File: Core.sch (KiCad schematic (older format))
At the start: 2 parts

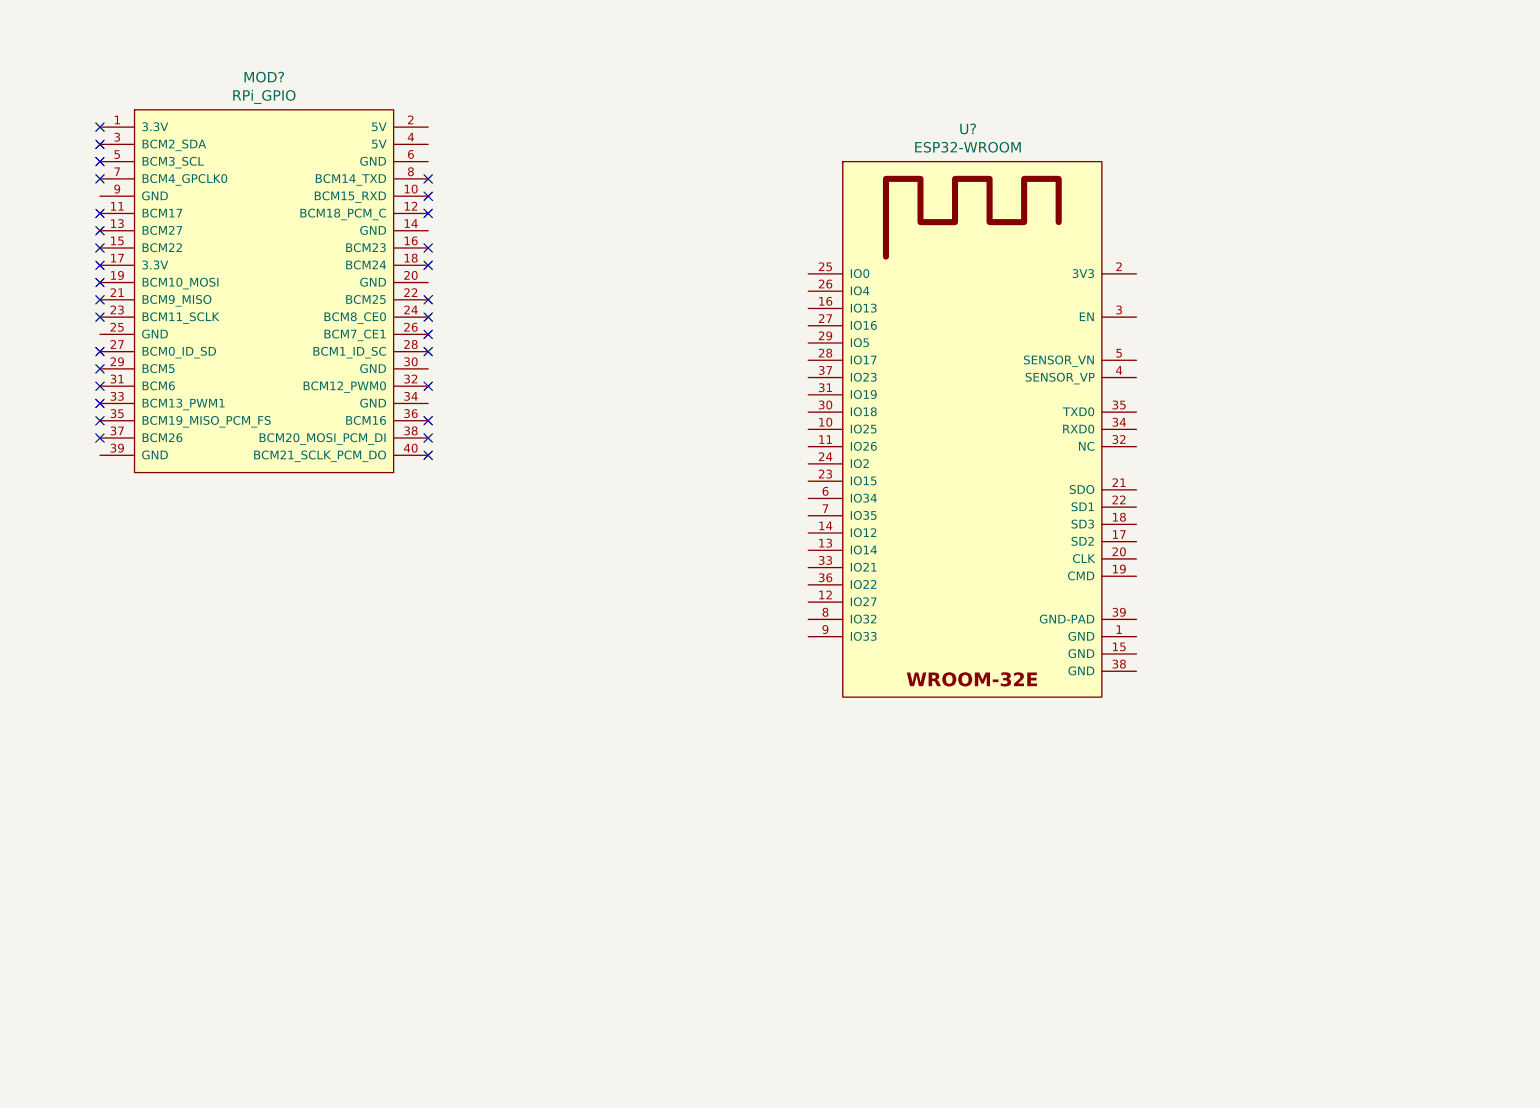
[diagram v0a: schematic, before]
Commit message: Agrego v1.0 de SmartSaffron
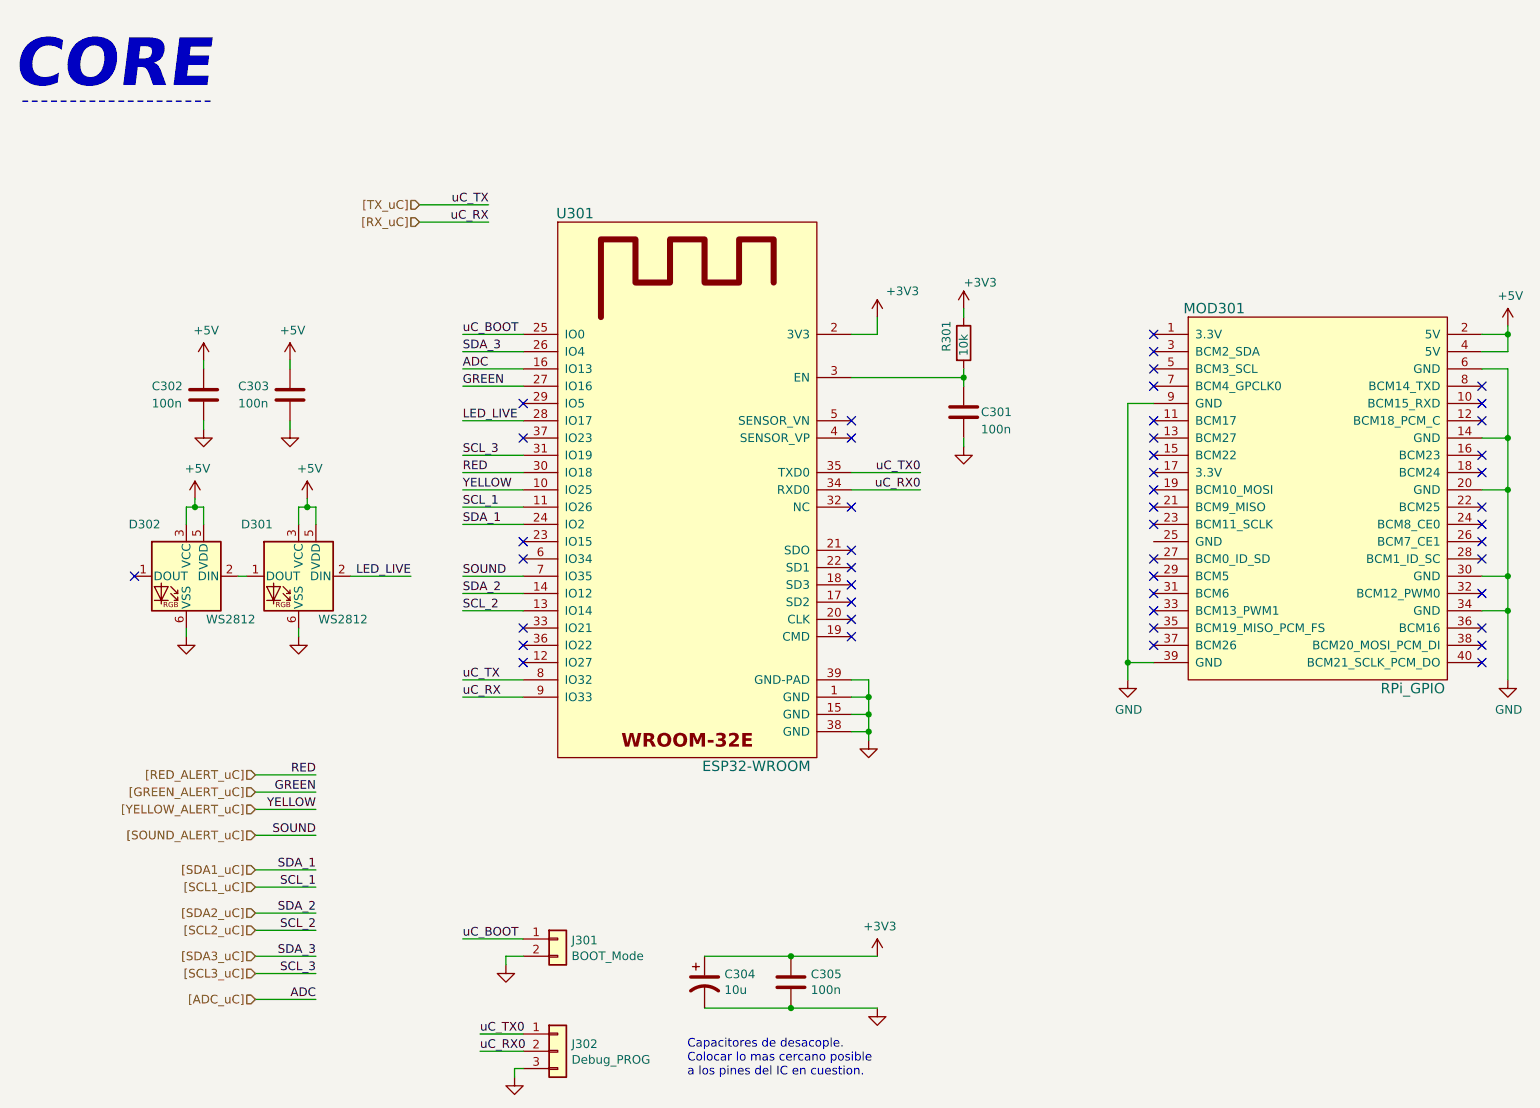
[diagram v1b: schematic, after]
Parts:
- added C301, C302, C303, C305: 100n, 00_lib_fp:C_0805_2012Metric_Pad1.18x1.45mm_HandSolder, symbol 00_lib_sch:C
- added C304: 10u, 00_lib_fp:C_0805_2012Metric_Pad1.18x1.45mm_HandSolder, symbol 00_lib_sch:CP1
- added D301, D302: WS2812, 00_lib_fp:LED_WS2812_PLCC6_5.0x5.0mm_P1.6mm, symbol 00_lib_sch:WS2812
- added J301: BOOT_Mode, 00_lib_fp:PinHeader_1x02_P2.54mm_Vertical, symbol 00_lib_sch:Conn_01x02
- added J302: Debug_PROG, 00_lib_fp:PinHeader_1x03_P2.54mm_Vertical, symbol Connector_Generic:Conn_01x03
- added R301: 10k, 00_lib_fp:R_0805_2012Metric_Pad1.20x1.40mm_HandSolder, symbol 00_lib_sch:R
- MOD301: renamed from MOD?; footprint 00_lib_fp:RPi_fp -> 00_lib_fp:PinSocket_2x20_P2.54mm_Vertical_SMD
- gave numbers to parts that had none: 1
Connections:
- net GND: now reaches MOD301.14 (GND)
- net GND: now also MOD301.20 (GND), MOD301.30 (GND), MOD301.34 (GND), MOD301.39 (GND), MOD301.6 (GND), MOD301.9 (GND), U301.1 (GND), U301.15 (GND), U301.38 (GND), U301.39 (GND-PAD), C301.2, C302.2, C303.2, C304.2, C305.2, D301.6 (VSS), D302.6 (VSS), J301.2 (Pin_2), J302.3 (Pin_3)
- net +5V: now reaches MOD301.2 (5V)
- net +5V: now also MOD301.4 (5V), C302.1, C303.1, D301.3 (VCC), D301.5 (VDD), D302.3 (VCC), D302.5 (VDD)
- net [YELLOW_ALERT_uC]: now reaches U301.10 (IO25)
- net [SCL1_uC]: now reaches U301.11 (IO26)
- net [SCL2_uC]: now reaches U301.13 (IO14)
- net [SDA2_uC]: now reaches U301.14 (IO12)
- net [ADC_uC]: now reaches U301.16 (IO13)
- net +3V3: now reaches U301.2 (3V3)
- net +3V3: now also C304.1, C305.1, R301.1
- net [SDA1_uC]: now reaches U301.24 (IO2)
- net uC_BOOT: now reaches U301.25 (IO0)
- net uC_BOOT: now also J301.1 (Pin_1)
- net [SDA3_uC]: now reaches U301.26 (IO4)
- net [GREEN_ALERT_uC]: now reaches U301.27 (IO16)
- net LED_LIVE: now reaches U301.28 (IO17)
- net LED_LIVE: now also D301.2 (DIN)
- net at U301.3 (EN): now also C301.1, R301.2
- net [RED_ALERT_uC]: now reaches U301.30 (IO18)
- net [SCL3_uC]: now reaches U301.31 (IO19)
- net uC_RX0: now reaches U301.34 (RXD0)
- net uC_RX0: now also J302.2 (Pin_2)
- net uC_TX0: now reaches U301.35 (TXD0)
- net uC_TX0: now also J302.1 (Pin_1)
- net [SOUND_ALERT_uC]: now reaches U301.7 (IO35)
- net [TX_uC]: now reaches U301.8 (IO32)
- net [RX_uC]: now reaches U301.9 (IO33)
- new net: D301.1 (DOUT), D302.2 (DIN)
- no-connect marks 30 -> 47
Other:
- note added: "CORE"
- note added: "Capacitores de desacople.\nColocar lo mas cercano posible \na los pines del IC en cuestion."
- moved on the sheet: MOD301, U301
